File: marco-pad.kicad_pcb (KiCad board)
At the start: 2 copper layers, 81.5 x 100 mm, 34 parts, among them SW1 SW_Push, SW10 SW_Push, SW11 SW_Push, SW12 SW_Push, SW13 SW_Push, SW14 SW_Push, SW15 SW_Push, SW16 SW_Push, SW2 SW_Push, SW3 SW_Push, SW4 SW_Push, SW5 SW_Push, SW6 SW_Push, SW7 SW_Push, SW8 SW_Push, SW9 SW_Push, U1 MOUDLE-SEEEDUINO-XIAO, U3 ER_OLEDM0.91_1x-I2C

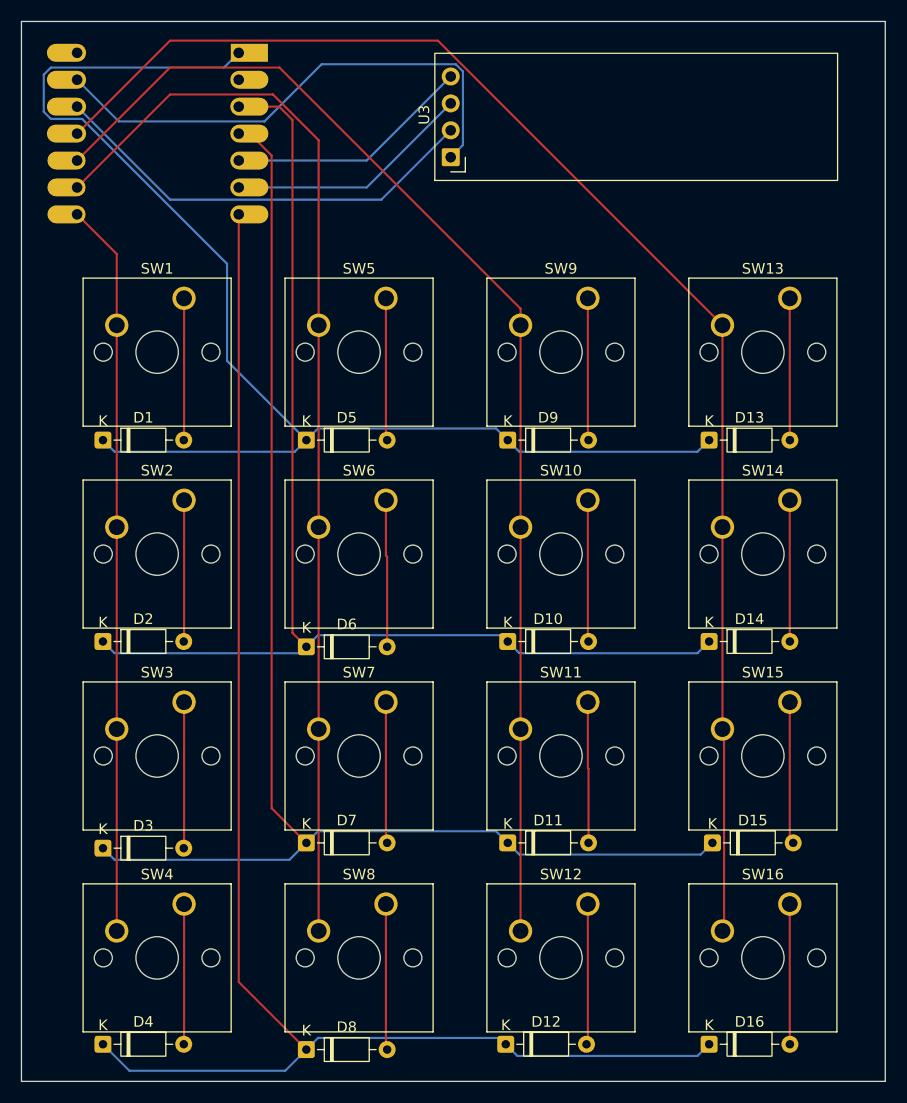
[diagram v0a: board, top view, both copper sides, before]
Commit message: Added Gerber files
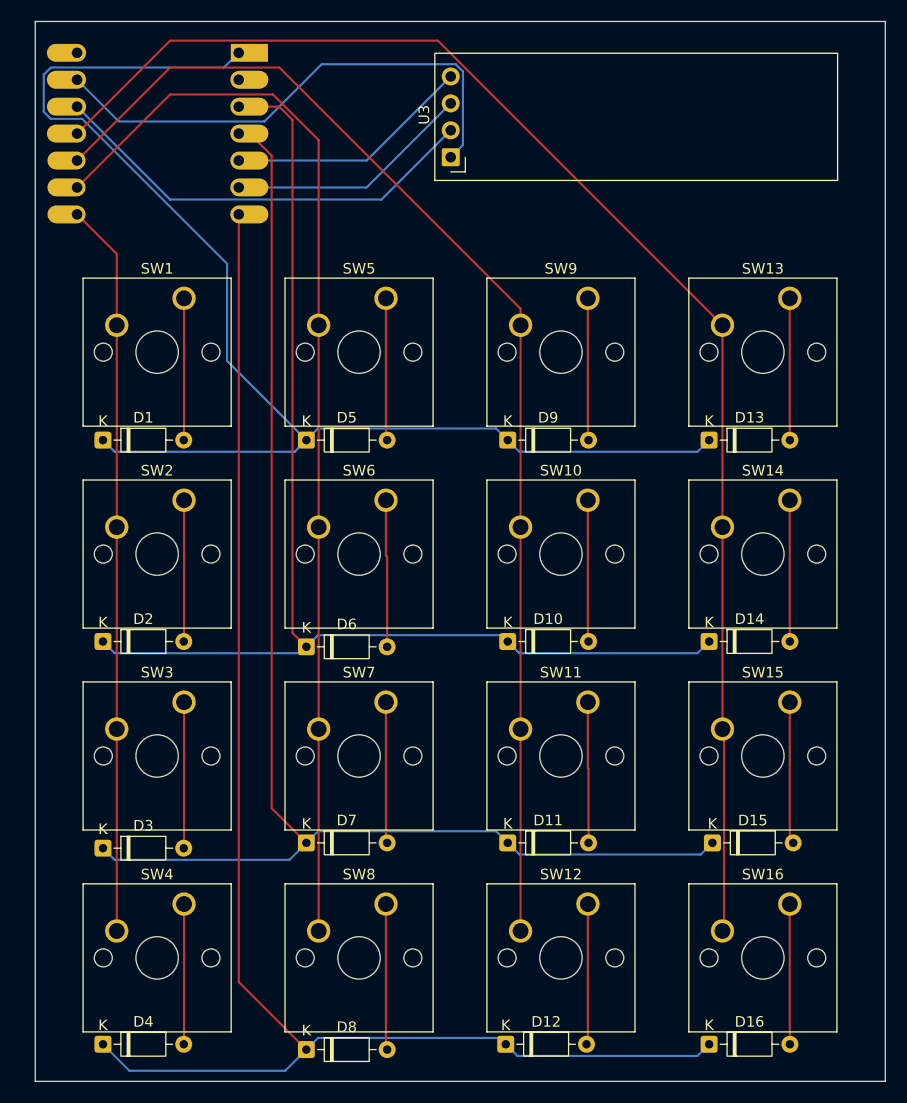
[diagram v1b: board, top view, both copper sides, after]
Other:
- board size 81.5 x 100 mm -> 80.2 x 100 mm
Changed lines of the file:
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@@
 			(outputformat 1)
 			(mirror no)
-			(drillshape 1)
+			(drillshape 0)
 			(scaleselection 1)
-			(outputdirectory "")
+			(outputdirectory "Gerber/")
 		)
 	)
@@
 	)
 	(gr_rect
-		(start 120.55 64.05)
+		(start 121.85 64.05)
 		(end 202.05 164.05)
 		(stroke
